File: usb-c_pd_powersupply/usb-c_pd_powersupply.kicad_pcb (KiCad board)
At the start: 2 copper layers, 72 parts, among them J1 USB_C_Receptacle, J2 TC2030-SWD, J3 Conn_01x02, J4 Conn_01x02, U1 STM32L011, U2 PTN5110, U3 AOZ1375DI, U4 LT3685, U5 LT3685, U6 LT3685, U7 CDSOT23-0502B

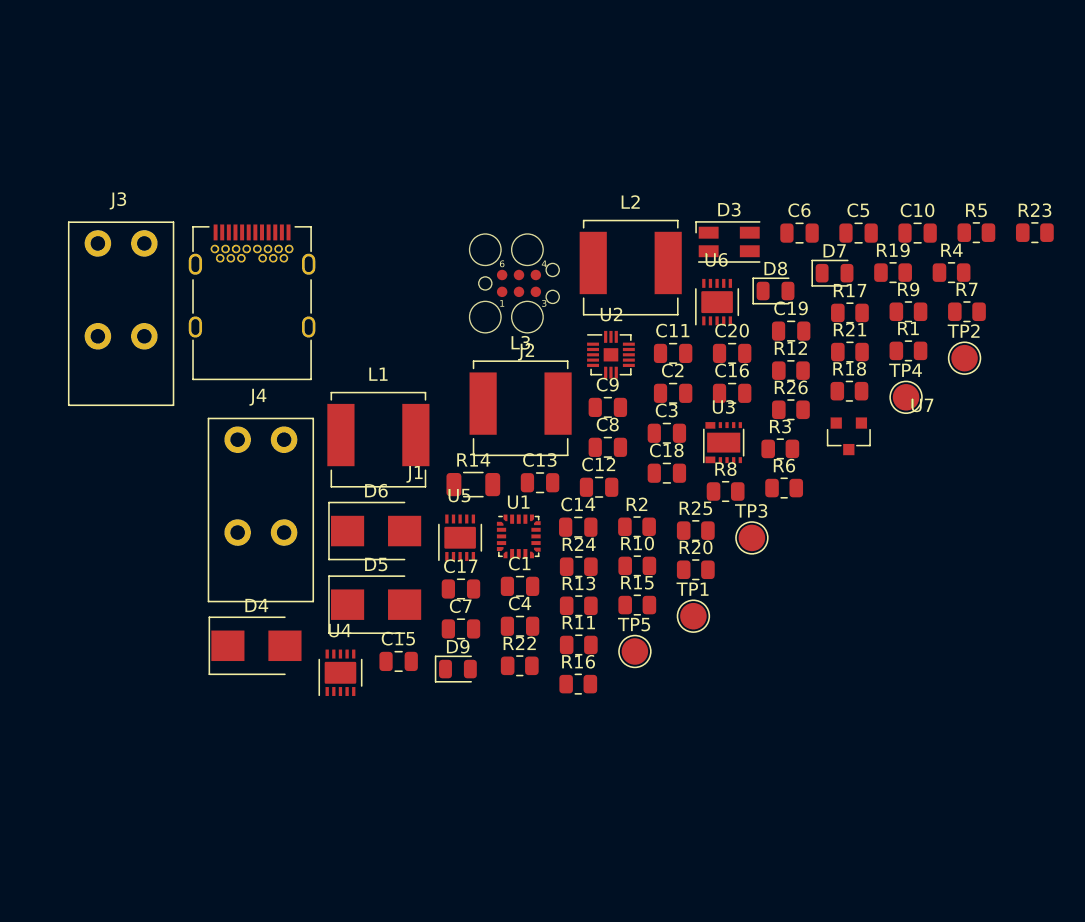
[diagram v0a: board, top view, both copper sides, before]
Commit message: Finished USB C PD Supply Layout
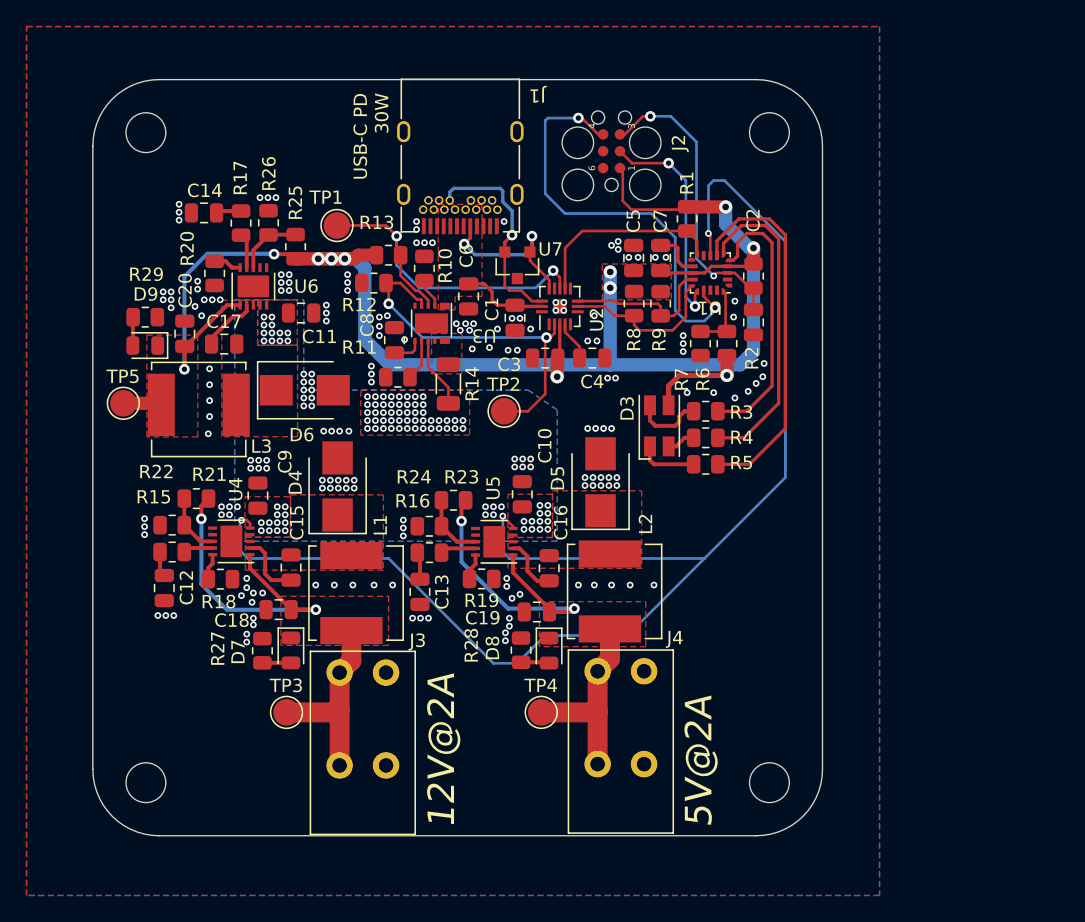
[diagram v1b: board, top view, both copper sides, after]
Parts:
- added R27: 500, Resistor_SMD:R_0805_2012Metric, F.Cu at (37.8, 67.1)
- added R28: 500, Resistor_SMD:R_0805_2012Metric, F.Cu at (57.3, 67.0)
- added R29: 500, Resistor_SMD:R_0805_2012Metric, F.Cu at (28.9, 41.9)
- added REF: MountingHole_3mm, MountingHole:MountingHole_3mm, F.Cu at (76.0, 77.0)
- added REF: MountingHole_3mm, MountingHole:MountingHole_3mm, F.Cu at (76.0, 28.0)
- added REF: MountingHole_3mm, MountingHole:MountingHole_3mm, F.Cu at (29.0, 77.0)
- added REF**: MountingHole_3mm, MountingHole:MountingHole_3mm, F.Cu at (29.0, 28.0)
- moved R21 50.5 mm to (32.8, 55.6)
- moved D7 49.9 mm to (39.9, 67.0), turned to -90 degrees
- moved R18 49.5 mm to (34.6, 61.7), turned to 180 degrees
- moved R23 48.2 mm to (52.2, 55.7)
- moved R17 46.4 mm to (36.2, 34.8), turned to -90 degrees
- moved TP5 42.9 mm to (27.3, 48.4)
- moved R20 42.6 mm to (34.2, 38.6), turned to 90 degrees
- moved R26 41.8 mm to (38.2, 34.8), turned to 90 degrees
- moved C20 41.3 mm to (31.9, 43.2), turned to 90 degrees
- moved TP1 39.9 mm to (43.4, 35.0)
- moved R19 38.7 mm to (54.3, 61.6), turned to 180 degrees
- moved TP3 37.5 mm to (39.6, 71.7)
- moved J3 37.1 mm to (43.6, 68.7)
- moved R25 37.0 mm to (40.3, 36.6), turned to -90 degrees
- moved C14 36.8 mm to (33.4, 34.0), turned to 180 degrees
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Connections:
- net Net-(C1-Pad2) renamed /VBUS
- net Net-(C10-Pad1) renamed /VBUS_SW
- net Net-(C15-Pad2) renamed /12V_SW
- net Net-(C16-Pad2) renamed /5V_SW
- net Net-(C17-Pad2) renamed /3V3_SW
- D7 pad 2: GND -> Net-(D7-Pad2)
- D8 pad 2: GND -> Net-(D8-Pad2)
- D9 pad 2: GND -> Net-(D9-Pad2)
- U1 pad 8: unconnected-(U1-Pad8) -> /OUT_EN
- U4 pad 5: unconnected-(U4-Pad5) -> /OUT_EN
- U5 pad 5: unconnected-(U5-Pad5) -> /OUT_EN
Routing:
- net +3V3: track 0.00 -> 123.9 mm, vias 0 -> 11
- net /OUT_EN: track 0.00 -> 104.2 mm, vias 0 -> 3
- net +12V: track 0.00 -> 38.0 mm, vias 0 -> 2
- net +5V: track 0.00 -> 37.0 mm, vias 0 -> 2
- net /SWDCLK: track 0.00 -> 32.7 mm, vias 0 -> 2
- net /IND_B: track 0.00 -> 28.3 mm
- net /VBUS_FAULT: track 0.00 -> 28.0 mm, vias 0 -> 2
- net /EN_SINK: track 0.00 -> 27.6 mm, vias 0 -> 2
- net /IND_G: track 0.00 -> 24.0 mm
- net /nRESET: track 0.00 -> 23.0 mm, vias 0 -> 2
- net /IND_R: track 0.00 -> 20.6 mm
- net /SWDIO: track 0.00 -> 16.9 mm, vias 0 -> 2
- net /CC2: track 0.00 -> 15.8 mm, vias 0 -> 1
- net /ALERT_N: track 0.00 -> 14.9 mm
- net /CC1: track 0.00 -> 12.6 mm, vias 0 -> 2
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- added copper zone on F.Cu, net +12V
- added copper zone on F.Cu, net +3V3
- added copper zone on F.Cu, net +5V
- added copper zone on F.Cu, net /12V_SW
- added copper zone on F.Cu, net /3V3_SW
- added copper zone on F.Cu, net /5V_SW
- added copper zone on F.Cu, net /VBUS
- added copper zone on B.Cu, net /VBUS_SW
- added copper zone on F.Cu, net /VBUS_SW
- added copper zone on B.Cu, net GND
- added copper zone on F.Cu, net GND
- added copper zone on In1.Cu, net GND
- added copper zone on In2.Cu, net GND
- added copper zone on F.Cu, net Net-(R14-Pad1)
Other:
- board outline added: 55 x 57 mm
- copper layers 2 -> 4
- board text added: "12V@2A"
- board text added: "5V@2A"
- board text added: "USB-C PD 30W"
- board text added: "USB-C PD Power Supply"
- board text added: "v1"
